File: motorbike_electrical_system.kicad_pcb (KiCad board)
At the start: 2 copper layers, 87.6 x 82.4 mm, 94 parts, among them IC3 BDX34C, IC4 BDX34C, IC5 BDX34C, IC6 BDX34C, Q1 D45VH10, Q2 D45VH10, U1 L7805, U2 L7805, U3 L7805

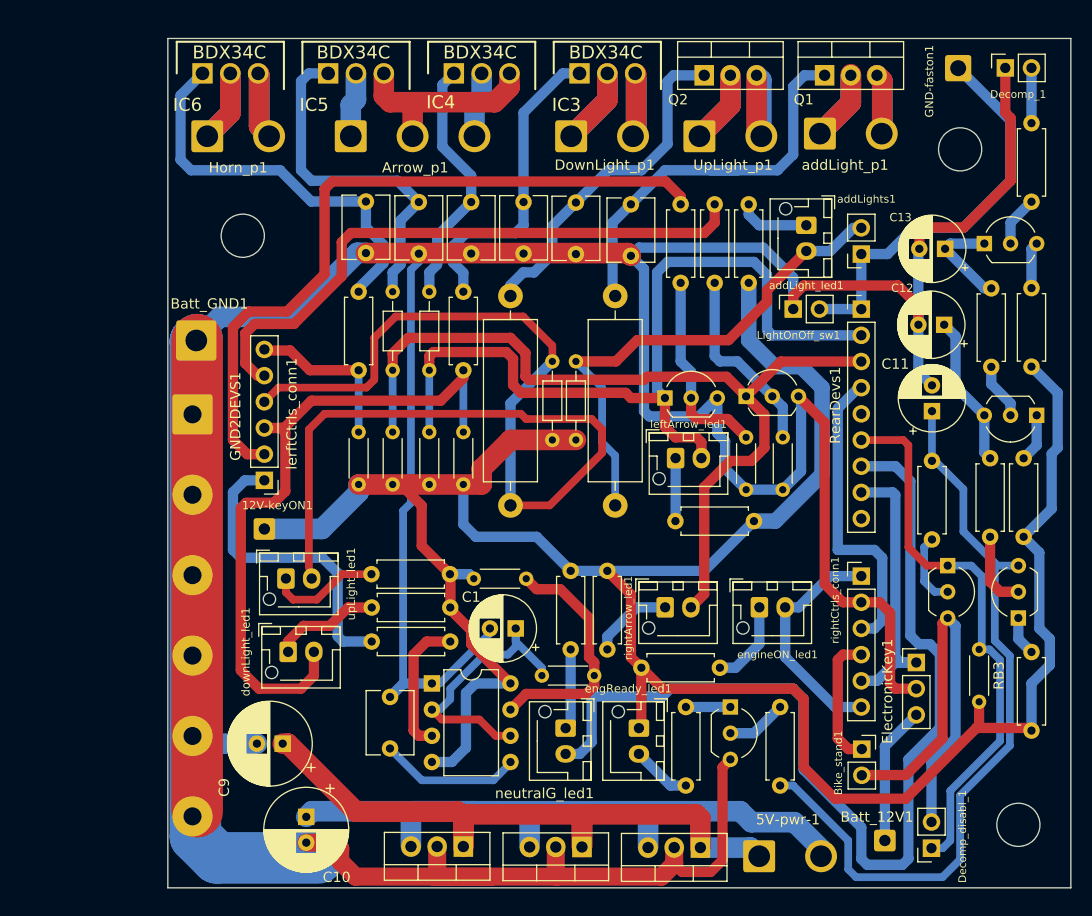
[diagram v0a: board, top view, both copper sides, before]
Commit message: First release of all-in-one solution
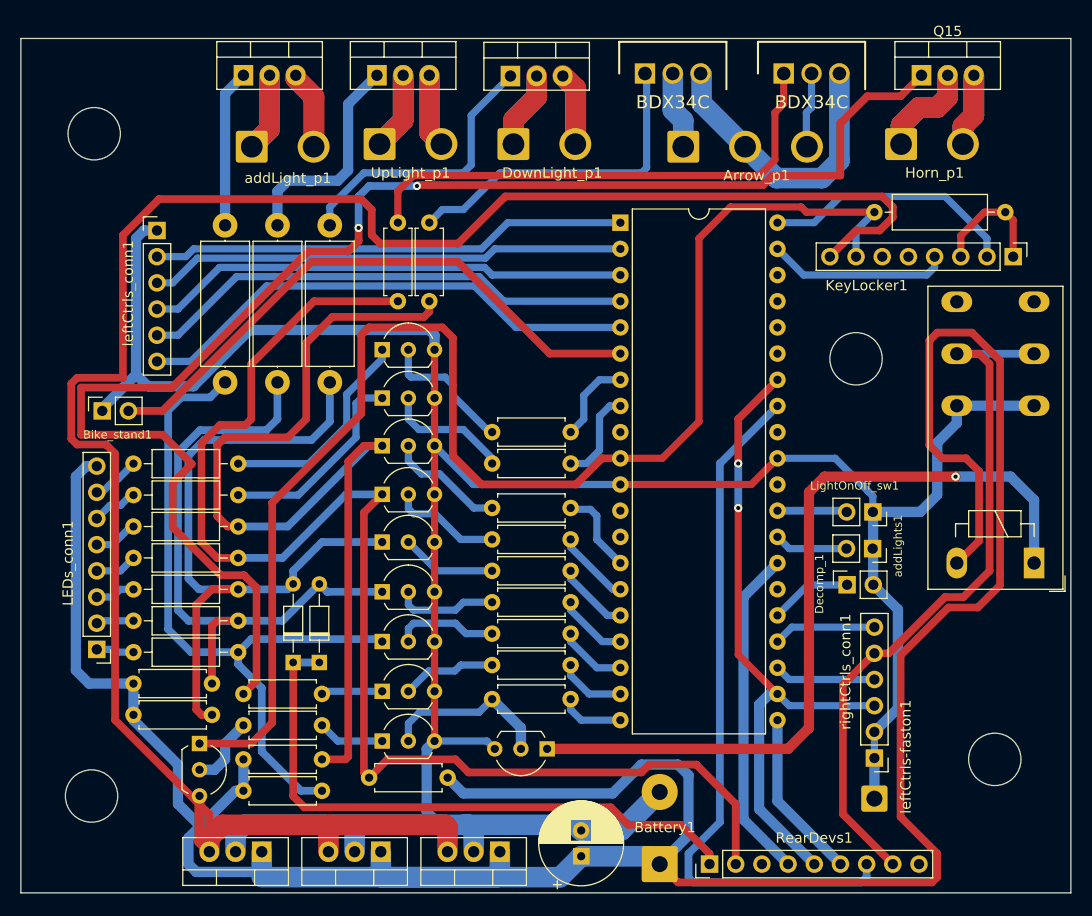
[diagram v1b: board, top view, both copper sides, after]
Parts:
- removed 12V-keyON1, Batt_12V1: Conn_01x01, Connector_Wire:SolderWire-0.5sqmm_1x01_D0.9mm_OD2.1mm
- removed 5V-pwr-1: Conn_01x02, Connector_Wire:SolderWire-1.5sqmm_1x02_P6mm_D1.7mm_OD3mm
- removed BT5, RB1, RB2, RB3, RBT2, RBT3, RBT4, RC1, RC2: 100K, Resistor_THT:R_Axial_DIN0204_L3.6mm_D1.6mm_P5.08mm_Horizontal
- removed Batt_GND1: Conn_01x01, Connector_Wire:SolderWire-1.5sqmm_1x01_D1.7mm_OD3.9mm
- removed C1: 1uF, Capacitor_THT:CP_Radial_D6.3mm_P2.50mm
- removed C10: C_Polarized_Small, Capacitor_THT:CP_Radial_D8.0mm_P2.50mm
- removed C11, C12, C13: 50uF, Capacitor_THT:CP_Radial_D6.3mm_P2.50mm
- removed C2, C3, C4, C5, C6, C7, C8: 100nf, Capacitor_THT:C_Disc_D6.0mm_W4.4mm_P5.00mm
- removed DC1: BC327, Package_TO_SOT_THT:TO-92_Inline_Wide
- removed DC2, DC3, DC4, DC5, Q_arr1, Q_arr2: BC337, Package_TO_SOT_THT:TO-92_Inline_Wide
- removed Decomp_disabl_1: Conn_01x02, Connector_PinSocket_2.54mm:PinSocket_1x02_P2.54mm_Vertical
- removed ElectronicKey1: Conn_01x03, Connector_PinHeader_2.54mm:PinHeader_1x03_P2.54mm_Vertical
- removed GND-faston1: Conn_01x01, Connector_Wire:SolderWire-0.75sqmm_1x01_D1.25mm_OD2.3mm
- removed GND2DEVS1: Conn_01x06, Connector_Wire:SolderWire-1sqmm_1x06_P7.8mm_D1.4mm_OD3.9mm
- removed IC4, IC5, IC6: BDX34C, BDX34C:TO270P460X1020X2008-3P
- removed RBT1, RBT6: 100K, Resistor_THT:R_Axial_DIN0204_L3.6mm_D1.6mm_P7.62mm_Horizontal
- removed RE1: 5K, Resistor_THT:R_Axial_DIN0207_L6.3mm_D2.5mm_P7.62mm_Horizontal
- removed RL1, RL10, RL2, RL3, RL4, RL5, RL6, RL7, RL8, RL9: 1.2K, Resistor_THT:R_Axial_DIN0207_L6.3mm_D2.5mm_P7.62mm_Horizontal
- removed RTA1, RTA6: 100, Resistor_THT:R_Axial_DIN0516_L15.5mm_D5.0mm_P20.32mm_Horizontal
- removed RTA2, RTA5: 2K, Resistor_THT:R_Axial_DIN0207_L6.3mm_D2.5mm_P7.62mm_Horizontal
- removed RTA3, RTA4: 8K, Resistor_THT:R_Axial_DIN0204_L3.6mm_D1.6mm_P7.62mm_Horizontal
- removed addLight_led1, downLight_led1, engReady_led1, engineON_led1, leftArrow_led1, neutralG_led1, rightArrow_led1, upLight_led1: Conn_01x02, Connector_JST:JST_XH_B2B-XH-AM_1x02_P2.50mm_Vertical
- removed lerftCtrls_conn1: Conn_01x06, Connector_PinHeader_2.54mm:PinHeader_1x06_P2.54mm_Vertical
- removed sqWaveGen1: NE555P, Package_DIP:DIP-8_W7.62mm
- added Battery1: Conn_01x02, Connector_Wire:SolderWire-0.75sqmm_1x02_P7mm_D1.25mm_OD3.5mm, F.Cu at (170.9, 135.8)
- added D1: DIODE, Diode_THT:D_DO-34_SOD68_P7.62mm_Horizontal, F.Cu at (135.4, 116.2)
- added D2: DIODE, Diode_THT:D_DO-34_SOD68_P7.62mm_Horizontal, F.Cu at (137.9, 116.2)
- added IC2: BDX34C, BDX34C:TO270P460X1020X2008-3P, F.Cu at (183.0, 59.1)
- added K1: RT42xxxx, Relay_THT:Relay_DPDT_Schrack-RT2-FormC_RM5mm, F.Cu at (207.3, 106.6)
- added KeyLocker1: Conn_01x08, Connector_PinHeader_2.54mm:PinHeader_1x08_P2.54mm_Vertical, F.Cu at (205.2, 76.8)
- added LEDs_conn1: Conn_01x08, Connector_PinHeader_2.54mm:PinHeader_1x08_P2.54mm_Vertical, F.Cu at (116.3, 115.0)
- added Q10: BC337, Package_TO_SOT_THT:TO-92L_Inline_Wide, F.Cu at (144.0, 85.9)
- added Q11: BC337, Package_TO_SOT_THT:TO-92L_Inline_Wide, F.Cu at (144.0, 123.8)
- added Q12: BC327, Package_TO_SOT_THT:TO-92L_Inline_Wide, F.Cu at (126.3, 124.1)
- added Q13: BC337, Package_TO_SOT_THT:TO-92L_Inline_Wide, F.Cu at (160.0, 124.6)
- added Q14: D45VH10, Package_TO_SOT_THT:TO-220-3_Vertical, F.Cu at (156.5, 59.3)
- added Q15: D45VH10, Package_TO_SOT_THT:TO-220-3_Vertical, F.Cu at (196.3, 59.3)
- added Q3: BC337, Package_TO_SOT_THT:TO-92L_Inline_Wide, F.Cu at (144.0, 114.2)
- added Q4: BC337, Package_TO_SOT_THT:TO-92L_Inline_Wide, F.Cu at (144.0, 109.4)
- added Q5: BC337, Package_TO_SOT_THT:TO-92L_Inline_Wide, F.Cu at (144.0, 104.5)
- added Q6: BC337, Package_TO_SOT_THT:TO-92L_Inline_Wide, F.Cu at (144.0, 99.9)
- added Q7: BC337, Package_TO_SOT_THT:TO-92L_Inline_Wide, F.Cu at (144.0, 95.2)
- added Q8: BC337, Package_TO_SOT_THT:TO-92L_Inline_Wide, F.Cu at (144.0, 90.6)
- added Q9: BC337, Package_TO_SOT_THT:TO-92L_Inline_Wide, F.Cu at (144.0, 119.0)
- added R1: 500, Resistor_THT:R_Axial_DIN0309_L9.0mm_D3.2mm_P12.70mm_Horizontal, F.Cu at (191.8, 72.5)
- added RA10: 240, Resistor_THT:R_Axial_DIN0414_L11.9mm_D4.5mm_P15.24mm_Horizontal, F.Cu at (128.8, 89.0)
- added RA11: 240, Resistor_THT:R_Axial_DIN0414_L11.9mm_D4.5mm_P15.24mm_Horizontal, F.Cu at (133.9, 89.0)
- added RA12: 240, Resistor_THT:R_Axial_DIN0414_L11.9mm_D4.5mm_P15.24mm_Horizontal, F.Cu at (138.9, 89.0)
- added RA13: 8K, Resistor_THT:R_Axial_DIN0207_L6.3mm_D2.5mm_P7.62mm_Horizontal, F.Cu at (145.6, 81.2)
- added RA14: 8K, Resistor_THT:R_Axial_DIN0207_L6.3mm_D2.5mm_P7.62mm_Horizontal, F.Cu at (148.6, 81.2)
- added RA15: 240, Resistor_THT:R_Axial_DIN0207_L6.3mm_D2.5mm_P7.62mm_Horizontal, F.Cu at (138.2, 119.3)
- added RA16: 5K, Resistor_THT:R_Axial_DIN0207_L6.3mm_D2.5mm_P7.62mm_Horizontal, F.Cu at (154.7, 93.9)
- added RA17: 5K, Resistor_THT:R_Axial_DIN0207_L6.3mm_D2.5mm_P7.62mm_Horizontal, F.Cu at (154.7, 96.9)
- added RA18: 5K, Resistor_THT:R_Axial_DIN0207_L6.3mm_D2.5mm_P7.62mm_Horizontal, F.Cu at (154.7, 101.2)
- added RA19: 5K, Resistor_THT:R_Axial_DIN0207_L6.3mm_D2.5mm_P7.62mm_Horizontal, F.Cu at (154.7, 104.3)
- added RA20: 5K, Resistor_THT:R_Axial_DIN0207_L6.3mm_D2.5mm_P7.62mm_Horizontal, F.Cu at (154.7, 107.3)
- added RA21: 5K, Resistor_THT:R_Axial_DIN0207_L6.3mm_D2.5mm_P7.62mm_Horizontal, F.Cu at (154.7, 110.4)
- added RA22: 5K, Resistor_THT:R_Axial_DIN0207_L6.3mm_D2.5mm_P7.62mm_Horizontal, F.Cu at (154.7, 113.4)
- added RA23: 5K, Resistor_THT:R_Axial_DIN0207_L6.3mm_D2.5mm_P7.62mm_Horizontal, F.Cu at (154.7, 116.5)
- added RA24: 100K, Resistor_THT:R_Axial_DIN0207_L6.3mm_D2.5mm_P7.62mm_Horizontal, F.Cu at (130.6, 128.7)
- added RA25: 100K, Resistor_THT:R_Axial_DIN0207_L6.3mm_D2.5mm_P7.62mm_Horizontal, F.Cu at (119.9, 118.3)
- added RA26: 100K, Resistor_THT:R_Axial_DIN0207_L6.3mm_D2.5mm_P7.62mm_Horizontal, F.Cu at (119.9, 121.3)
- added RA27: 100K, Resistor_THT:R_Axial_DIN0207_L6.3mm_D2.5mm_P7.62mm_Horizontal, F.Cu at (150.4, 127.4)
- added RA28: 100K, Resistor_THT:R_Axial_DIN0207_L6.3mm_D2.5mm_P7.62mm_Horizontal, F.Cu at (130.6, 125.6)
- added RA9: 0, Resistor_THT:R_Axial_DIN0207_L6.3mm_D2.5mm_P10.16mm_Horizontal, F.Cu at (130.1, 96.9)
- added U4: ATmega16L-8P, Package_DIP:DIP-40_W15.24mm, F.Cu at (167.1, 73.6)
- added leftCtrls-faston1: Conn_01x01, Connector_Wire:SolderWire-0.75sqmm_1x01_D1.25mm_OD2.3mm, F.Cu at (191.8, 129.4)
- added leftCtrls_conn1: Conn_01x06, Connector_PinHeader_2.54mm:PinHeader_1x06_P2.54mm_Vertical, F.Cu at (122.2, 74.3)
- RA1, RA2: value 5K -> 0; footprint Resistor_THT:R_Axial_DIN0207_L6.3mm_D2.5mm_P7.62mm_Horizontal -> Resistor_THT:R_Axial_DIN0207_L6.3mm_D2.5mm_P10.16mm_Horizontal
- RA3, RA5: value 12K -> 0; footprint Resistor_THT:R_Axial_DIN0207_L6.3mm_D2.5mm_P7.62mm_Horizontal -> Resistor_THT:R_Axial_DIN0207_L6.3mm_D2.5mm_P10.16mm_Horizontal
- RA4, RA6: value 24K -> 0; footprint Resistor_THT:R_Axial_DIN0207_L6.3mm_D2.5mm_P7.62mm_Horizontal -> Resistor_THT:R_Axial_DIN0207_L6.3mm_D2.5mm_P10.16mm_Horizontal
- RA7: value 1.2K -> 1K
- RA8: value 24K -> 3K
- moved Bike_stand1 80.7 mm to (116.9, 91.8), turned to 90 degrees
- moved RA8 76.6 mm to (154.7, 119.8), turned to 0 degrees
- moved RA6 75.8 mm to (130.1, 100.0), turned to 180 degrees
- moved RA4 73.6 mm to (130.1, 106.1), turned to 180 degrees
- moved RA3 68.5 mm to (130.1, 109.1), turned to 180 degrees
- moved Horn_p1 67.3 mm to (194.4, 65.9)
- moved RA2 56.7 mm to (130.1, 112.2), turned to 180 degrees
- moved Q1 56.4 mm to (130.6, 59.3)
- moved RA1 55.9 mm to (130.1, 115.2), turned to 180 degrees
- moved RearDevs1 55.8 mm to (175.8, 135.8), turned to 90 degrees
- moved RA5 55.4 mm to (130.1, 103.0), turned to 180 degrees
- moved addLight_p1 55.1 mm to (131.4, 66.2)
- moved Decomp_1 52.4 mm to (189.1, 108.7)
- moved RA7 35.8 mm to (138.2, 122.3), turned to 180 degrees
- moved Arrow_p1 32.3 mm to (173.2, 66.2)
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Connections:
- net Net-(5V-pwr-1-Pad2) renamed +5V
- net Net-(ElectronicKey1-Pad1) renamed c_engineOFF
- Bike_stand1 pad 1: Net-(Bike_stand1-Pad1) -> GND
- Bike_stand1 pad 2: Net-(Bike_stand1-Pad2) -> i_bykeStand
- C9 pad 1: Net-(5V-pwr-1-Pad1) -> +12V
- Decomp_1 pad 1: GND -> i_decompr
- Decomp_1 pad 2: Net-(Decomp_1-Pad2) -> GND
- IC3 pad 2: Net-(DownLight_p1-Pad1) -> Net-(Arrow_p1-Pad1)
- IC3 pad 3: Net-(DownLight_p1-Pad2) -> Net-(Arrow_p1-Pad2)
- LightOnOff_sw1 pad 2: Net-(GND-faston1-Pad1) -> i_lightON/OFF
- RA3 pad 1: Net-(C11-Pad1) -> Net-(D1-Pad2)
- RA4 pad 1: Net-(C12-Pad1) -> c_leftArrow
- RA5 pad 2: Net-(C11-Pad1) -> Net-(LEDs_conn1-Pad5)
- RA8 pad 1: Net-(Decomp_1-Pad2) -> Net-(Q11-Pad2)
- RA8 pad 2: Net-(DC1-Pad2) -> o_keepAlive
- RearDevs1 pad 1: Net-(GND-faston1-Pad1) -> c_rearLight
- RearDevs1 pad 2: Net-(Q_arr1-Pad1) -> c_leftArrow
- RearDevs1 pad 3: Net-(Q_arr2-Pad1) -> c_rightArrow
- RearDevs1 pad 4: Net-(RearDevs1-Pad4) -> o_stopLight
- RearDevs1 pad 5: unconnected-(RearDevs1-Pad5) -> i_brakeSwitch
- RearDevs1 pad 6: Net-(DC4-Pad1) -> o_startEngine
- RearDevs1 pad 7: Net-(RearDevs1-Pad7) -> i_neutral
- U1 pad 1: Net-(5V-pwr-1-Pad1) -> +12V
- U2 pad 1: Net-(5V-pwr-1-Pad1) -> +12V
- U3 pad 1: Net-(5V-pwr-1-Pad1) -> +12V
- addLights1 pad 1: Net-(GND-faston1-Pad1) -> GND
- addLights1 pad 2: Net-(RBT6-Pad2) -> i_addLight
- rightCtrls_conn1 pad 1: Net-(engineON_led1-Pad2) -> GND
- rightCtrls_conn1 pad 3: Net-(RearDevs1-Pad4) -> i_brakeSwitch
- rightCtrls_conn1 pad 4: Net-(Bike_stand1-Pad1) -> i_startButton
- rightCtrls_conn1 pad 6: Net-(engineON_led1-Pad2) -> i_engineON
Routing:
- net GND: track 439.9 -> 259.5 mm
- net Net-(Q15-Pad1): track 0.00 -> 144.4 mm, vias 0 -> 2
- net tempPower: track 0.00 -> 139.0 mm
- net c_leftArrow: track 0.00 -> 131.2 mm
- net +5V: track 74.2 -> 198.0 mm
- net Net-(RBT1-Pad2): track 107.8 -> 0.00 mm
- net Net-(RearDevs1-Pad7): track 96.5 -> 0.00 mm
- net Net-(Q7-Pad1): track 5.88 -> 93.0 mm
- net Net-(Q_arr2-Pad1): track 84.4 -> 0.00 mm
- net Net-(Q_arr1-Pad1): track 81.0 -> 0.00 mm
- net Net-(K1-PadA1): track 0.00 -> 78.6 mm, vias 0 -> 1
- net Net-(C11-Pad1): track 74.4 -> 0.00 mm
- net Net-(D1-Pad2): track 0.00 -> 69.3 mm
- net i_neutral: track 0.00 -> 68.3 mm
- net Net-(RBT2-Pad2): track 67.4 -> 0.00 mm
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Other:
- board size 87.6 x 82.4 mm -> 101.9 x 82.9 mm
